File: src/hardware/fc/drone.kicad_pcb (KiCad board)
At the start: 4 copper layers, 40 x 40 mm, 138 parts, among them J1 Conn_01x01, J10 Conn_01x01, J11 Conn_01x01, J12 Micro_SD_Card, J13 Conn_01x01, J14 Conn_01x01, J15 Conn_01x01, J16 Conn_01x01, J17 Conn_01x01, J18 Conn_01x01, J19 Conn_01x03, J2 Conn_01x08, J20 Conn_01x03, J21 Conn_01x03, J22 Conn_01x03, J23 Conn_01x01, J24 Conn_01x01, J25 Conn_01x01, J26 Conn_01x01, J27 Conn_01x01, J28 Conn_01x01, J29 Conn_01x01, J3 Conn_01x01, J4 Conn_01x01, J5 Conn_01x01, J6 Conn_01x01, J7 Conn_01x01, J8 Conn_01x01, J9 Conn_01x01, Q1 AO3400A, Q2 NPN, SW1 SW_Push, SW2 SW_Push, U1 MP9943GQ(TOKMAS), U10 LM66100DCK, U2 TLV75533PDBV, U3 W25Q128JVP, U4 RP2350_80QFN, U5 ICM-42688-P, U6 LP5907MFX-3.3, U7 MP9943GQ(TOKMAS), U8 BMP280, U9 LM66100DCK, Y1 ABM8-272-T3

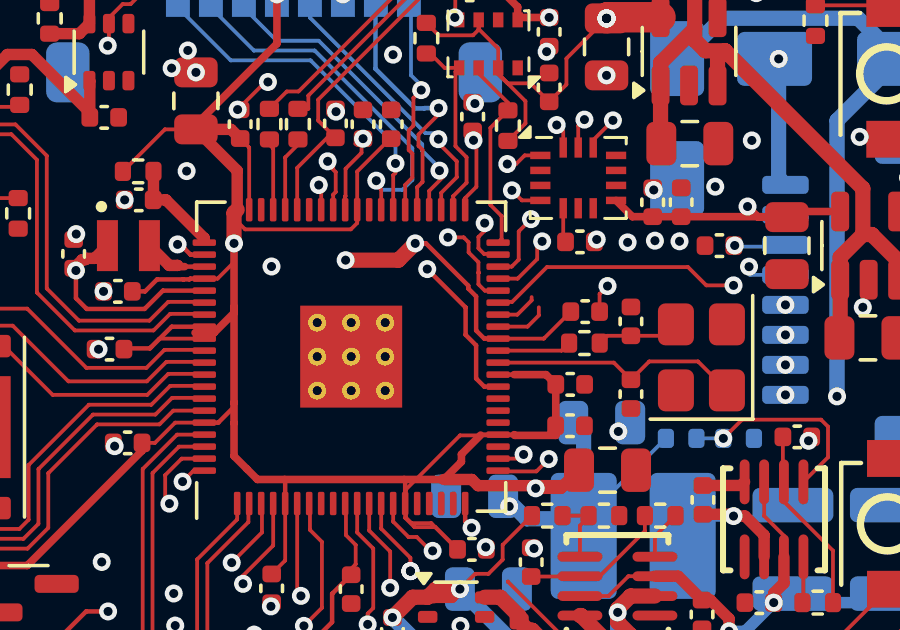
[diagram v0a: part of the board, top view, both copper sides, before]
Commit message: poush up to date
its been a long time since i last pushed but some updates were on the way
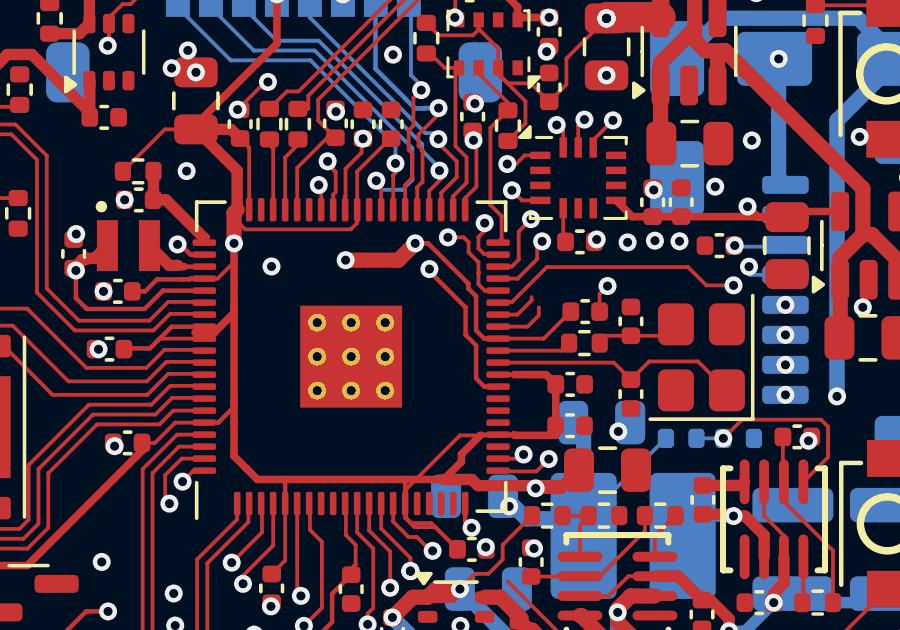
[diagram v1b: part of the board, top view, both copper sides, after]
